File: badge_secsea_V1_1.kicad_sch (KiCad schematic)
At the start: 132 parts, among them J1 USB_C_Receptacle_USB2.0_14P, J4 AFC07-S24ECA-00, J5 Micro_SD_Card_Det1, Q1 2N7002, Q2 SI1308EDL, Q3 SI2301, SW1 TS-1187A-B-A-B, SW2 K2-1112SW-A4SW-04, SW3 K2-1112SW-A4SW-04, SW4 XDTD-6650, SW5 XDTD-6650, SW6 TS-1187A-B-A-B, SW7 SW_SPDT, U1 RP2040, U2 74HC139, U3 W25Q128JVSIQ, U4 CC1101RGPR, U5 TP4056, U6 TPS63000, U7 LM321, X1 ABM8-272-T3, X2 26MHz

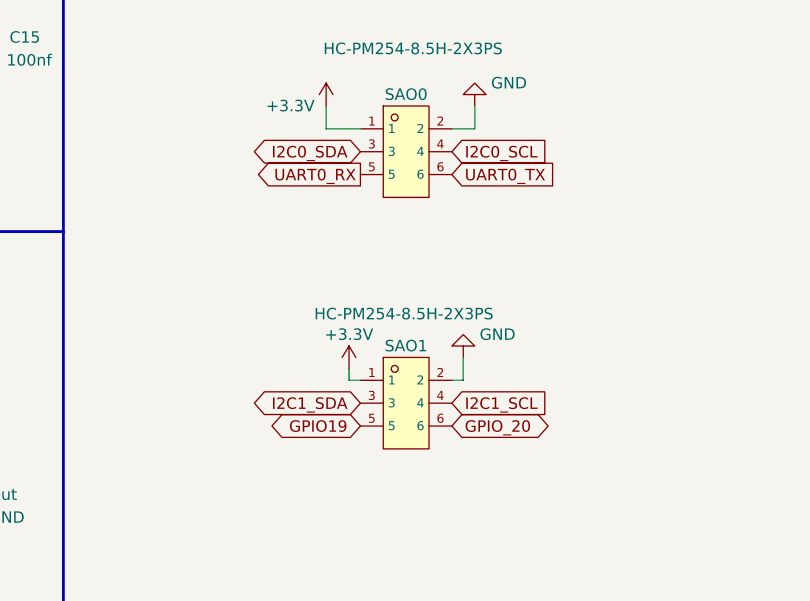
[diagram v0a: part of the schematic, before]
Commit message: WIP Routing....
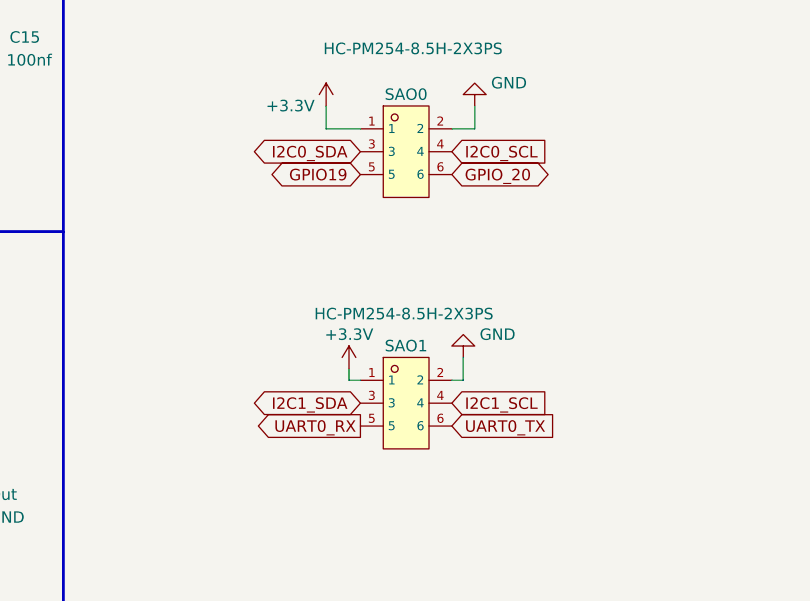
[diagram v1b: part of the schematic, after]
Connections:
- net GPIO19: now also SAO0.5; no longer SAO1.5
- net GPIO_20: now also SAO0.6; no longer SAO1.6
- net UART0_RX: now also SAO1.5; no longer SAO0.5
- net UART0_TX: now also SAO1.6; no longer SAO0.6
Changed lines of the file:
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@@
 	(global_label "UART0_RX"
 		(shape output)
-		(at 405.13 280.67 180)
-		(effects
-			(font
-				(size 1.27 1.27)
-			)
-			(justify right)
-		)
-		(property "Intersheetrefs" "${INTERSHEET_REFS}"
-			(at 405.13 280.67 0)
+		(at 405.13 308.61 180)
+		(effects
+			(font
+				(size 1.27 1.27)
+			)
+			(justify right)
+		)
+		(property "Intersheetrefs" "${INTERSHEET_REFS}"
+			(at 405.13 308.61 0)
 			(hide yes)
 			(show_name no)
@@
 	(global_label "GPIO19"
 		(shape bidirectional)
-		(at 405.13 308.61 180)
-		(effects
-			(font
-				(size 1.27 1.27)
-			)
-			(justify right)
-		)
-		(property "Intersheetrefs" "${INTERSHEET_REFS}"
-			(at 405.13 308.61 0)
+		(at 405.13 280.67 180)
+		(effects
+			(font
+				(size 1.27 1.27)
+			)
+			(justify right)
+		)
+		(property "Intersheetrefs" "${INTERSHEET_REFS}"
+			(at 405.13 280.67 0)
 			(hide yes)
 			(show_name no)
@@
 	(global_label "GPIO_20"
 		(shape bidirectional)
-		(at 415.29 308.61 0)
-		(effects
-			(font
-				(size 1.27 1.27)
-			)
-			(justify left)
-		)
-		(property "Intersheetrefs" "${INTERSHEET_REFS}"
-			(at 415.29 308.61 0)
+		(at 415.29 280.67 0)
+		(effects
+			(font
+				(size 1.27 1.27)
+			)
+			(justify left)
+		)
+		(property "Intersheetrefs" "${INTERSHEET_REFS}"
+			(at 415.29 280.67 0)
 			(hide yes)
 			(show_name no)
@@
 	(global_label "UART0_TX"
 		(shape input)
-		(at 415.29 280.67 0)
-		(effects
-			(font
-				(size 1.27 1.27)
-			)
-			(justify left)
-		)
-		(property "Intersheetrefs" "${INTERSHEET_REFS}"
-			(at 415.29 280.67 0)
-			(hide yes)
-			(show_name no)
+		(at 415.29 308.61 0)
+		(effects
+			(font
+				(size 1.27 1.27)
+			)
+			(justify left)
+		)
+		(property "Intersheetrefs" "${INTERSHEET_REFS}"
+			(at 415.29 308.61 0)
+			(hide yes)
+			(show_name no)
